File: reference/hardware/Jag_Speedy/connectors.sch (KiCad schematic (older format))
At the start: 8 parts, among them J1 Inputs, J2 Ouputs01, J3 Outputs02, J4 Power, J5 Bluetooth, J7 Canbus, U5 SN65HVD230

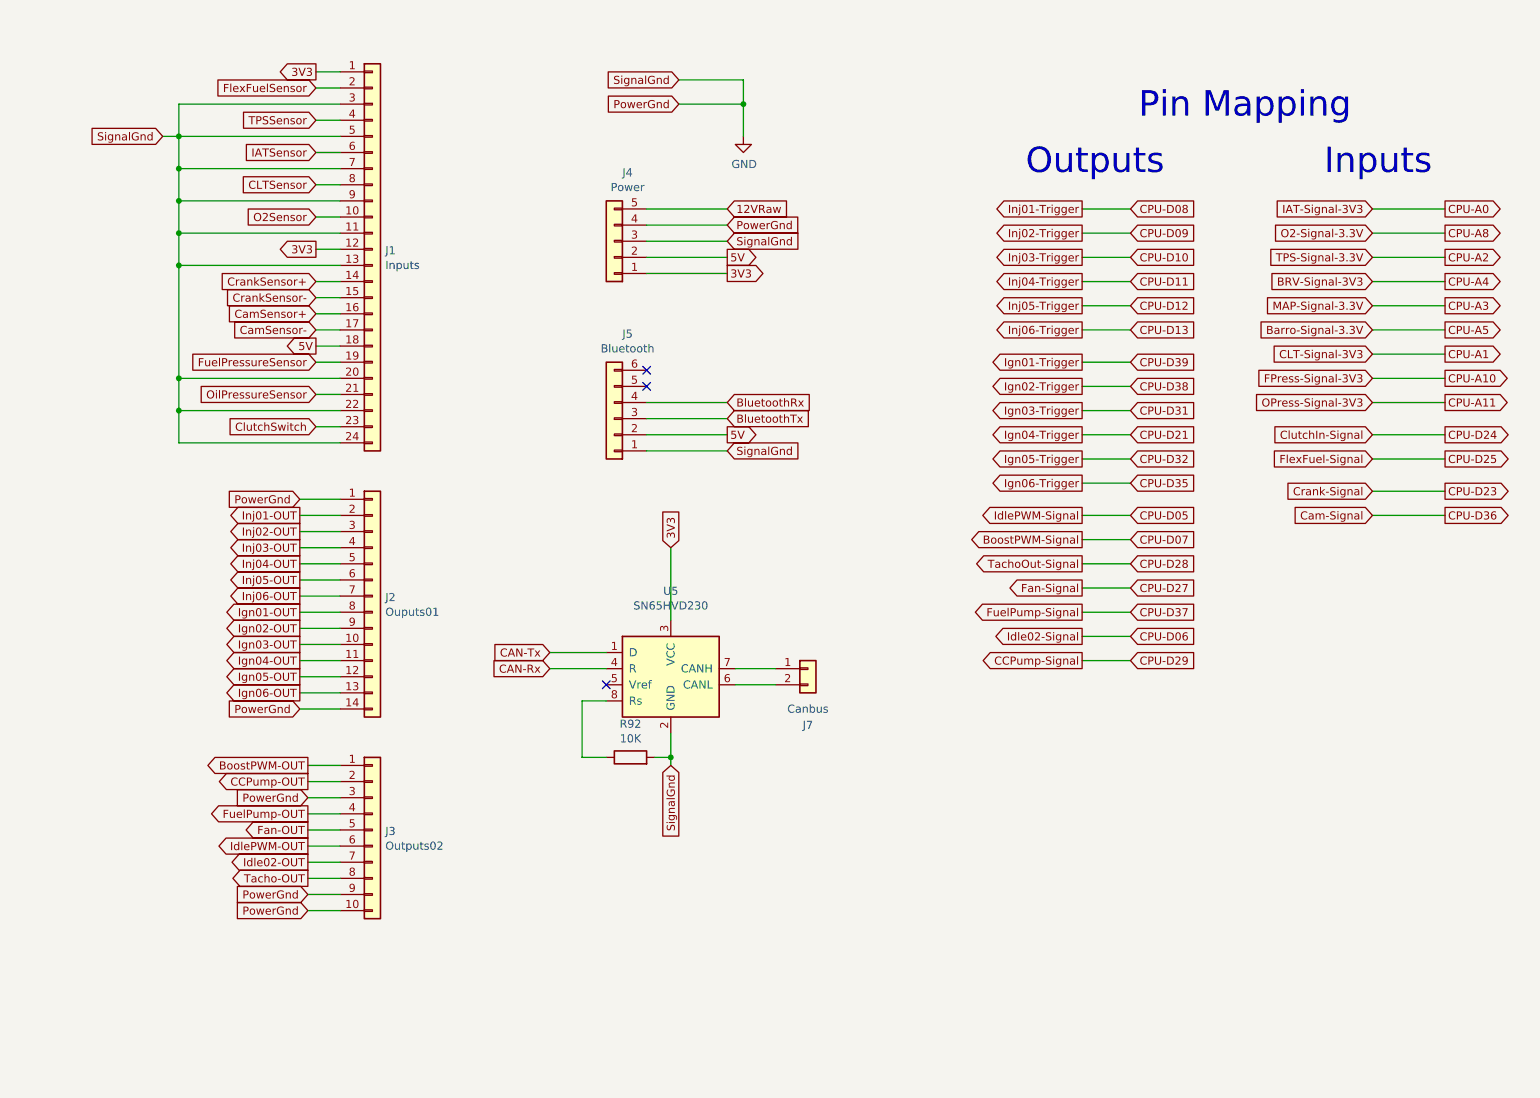
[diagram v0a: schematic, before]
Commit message: Connector update
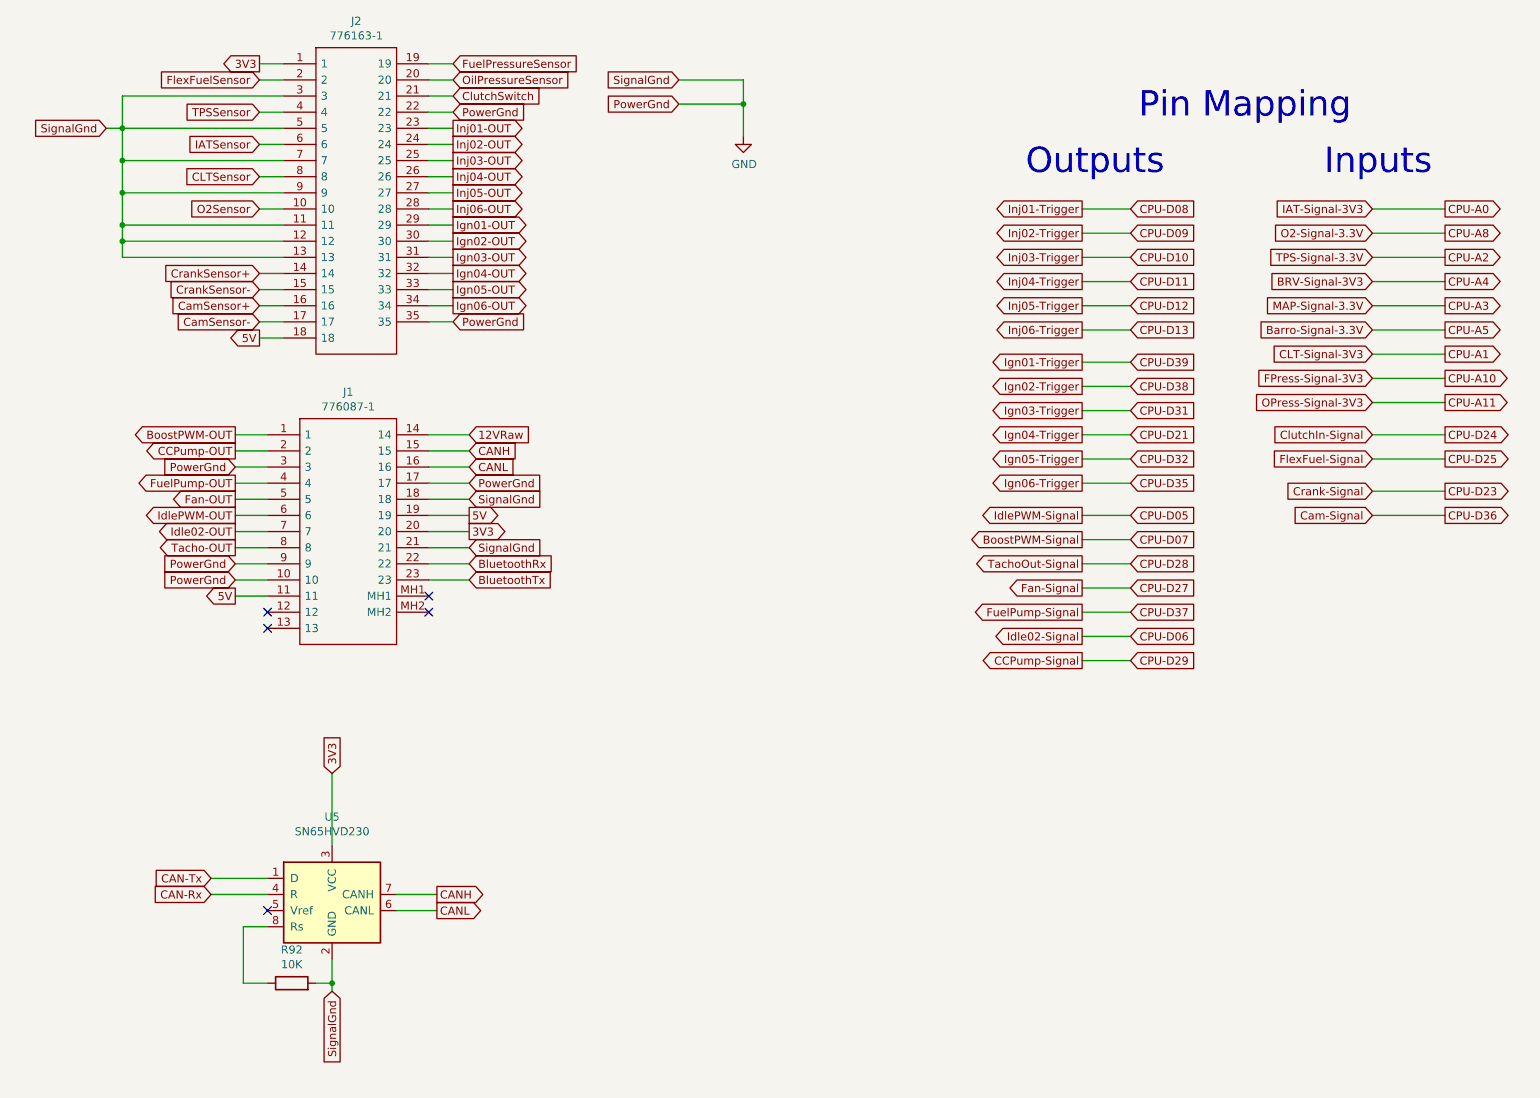
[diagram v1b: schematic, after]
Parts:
- removed J1: Inputs, Connector_PinHeader_1.00mm:PinHeader_2x12_P1.00mm_Horizontal, symbol Connector_Generic:Conn_01x24
- removed J2: Ouputs01, Connector_PinHeader_1.00mm:PinHeader_2x07_P1.00mm_Horizontal, symbol Connector_Generic:Conn_01x14
- removed J3: Outputs02, Connector_PinHeader_1.00mm:PinHeader_2x05_P1.00mm_Horizontal, symbol Connector_Generic:Conn_01x10
- removed J4: Power, Connector_PinHeader_1.00mm:PinHeader_1x05_P1.00mm_Horizontal, symbol Connector_Generic:Conn_01x05
- removed J5: Bluetooth, Connector_PinHeader_1.00mm:PinHeader_1x06_P1.00mm_Horizontal, symbol Connector_Generic:Conn_01x06
- removed J7: Canbus, Connector_PinHeader_1.00mm:PinHeader_1x06_P1.00mm_Horizontal, symbol Connector_Generic:Conn_01x02
- added J1: 776087-1, 776087-1:7760871, symbol 776087-1:776087-1
- added J2: 776163-1, 776163-1:776163-1, symbol 776163-1:776163-1
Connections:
- net 12VRaw: now also J1.14
- net 3V3: now also J1.20, J2.1
- net 5V: now also J1.11, J1.19, J2.18
- net BluetoothRx: now also J1.22
- net BluetoothTx: now also J1.23
- net BoostPWM-OUT: now also J1.1
- net CCPump-OUT: now also J1.2
- net CLTSensor: now also J2.8
- net CamSensor+: now also J2.16
- net CamSensor-: now also J2.17
- net ClutchSwitch: now also J2.21
- net CrankSensor+: now also J2.14
- net CrankSensor-: now also J2.15
- net Fan-OUT: now also J1.5
- net FlexFuelSensor: now also J2.2
- net FuelPressureSensor: now also J2.19
- net FuelPump-OUT: now also J1.4
- net GND: now also J1.10, J1.17, J1.18, J1.21, J1.3, J1.9, J2.11, J2.12, J2.13, J2.22, J2.3, J2.35, J2.5, J2.7, J2.9
- net IATSensor: now also J2.6
- net Idle02-OUT: now also J1.7
- net IdlePWM-OUT: now also J1.6
- net Ign01-OUT: now also J2.29
- net Ign02-OUT: now also J2.30
- net Ign03-OUT: now also J2.31
- net Ign04-OUT: now also J2.32
- net Ign05-OUT: now also J2.33
- net Ign06-OUT: now also J2.34
- net Inj01-OUT: now also J2.23
- net Inj02-OUT: now also J2.24
- net Inj03-OUT: now also J2.25
- net Inj04-OUT: now also J2.26
- net Inj05-OUT: now also J2.27
- net Inj06-OUT: now also J2.28
- net O2Sensor: now also J2.10
- net OilPressureSensor: now also J2.20
- net TPSSensor: now also J2.4
- net Tacho-OUT: now also J1.8
- net CANL: now reaches U5.6 (CANL)
- net CANL: now also J1.16
- net CANH: now reaches U5.7 (CANH)
- net CANH: now also J1.15
- no-connect marks 3 -> 5
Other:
- moved on the sheet: R92, U5
